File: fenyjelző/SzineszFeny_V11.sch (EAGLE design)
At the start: 203 parts, among them CN3 PIN05_2'THT', IC1 BEM_VEDO, IC2 BEM_VEDO, IC3 BEM_VEDO, IC4 BEM_VEDO, IC5 BEM_VEDO, IC6 BEM_VEDO, IC7 SCT2168SOP16, IC8 SCT2168SOP16, IC9 SCT2168SOP16, U1 MICROCHIP_PIC18F45K80-I-MLMIC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, U10 AP2625GY-HF-3SOT26, U11 AP2625GY-HF-3SOT26, U12 AP2625GY-HF-3SOT26, U13 AP2625GY-HF-3SOT26, U14 AP2625GY-HF-3SOT26, U15 AP2625GY-HF-3SOT26, U16 FDC6306P, U5 FDC6306P, U6 AP2625GY-HF-3SOT26, U7 AP2625GY-HF-3SOT26, U8 AP2625GY-HF-3SOT26, U9 AP2625GY-HF-3SOT26

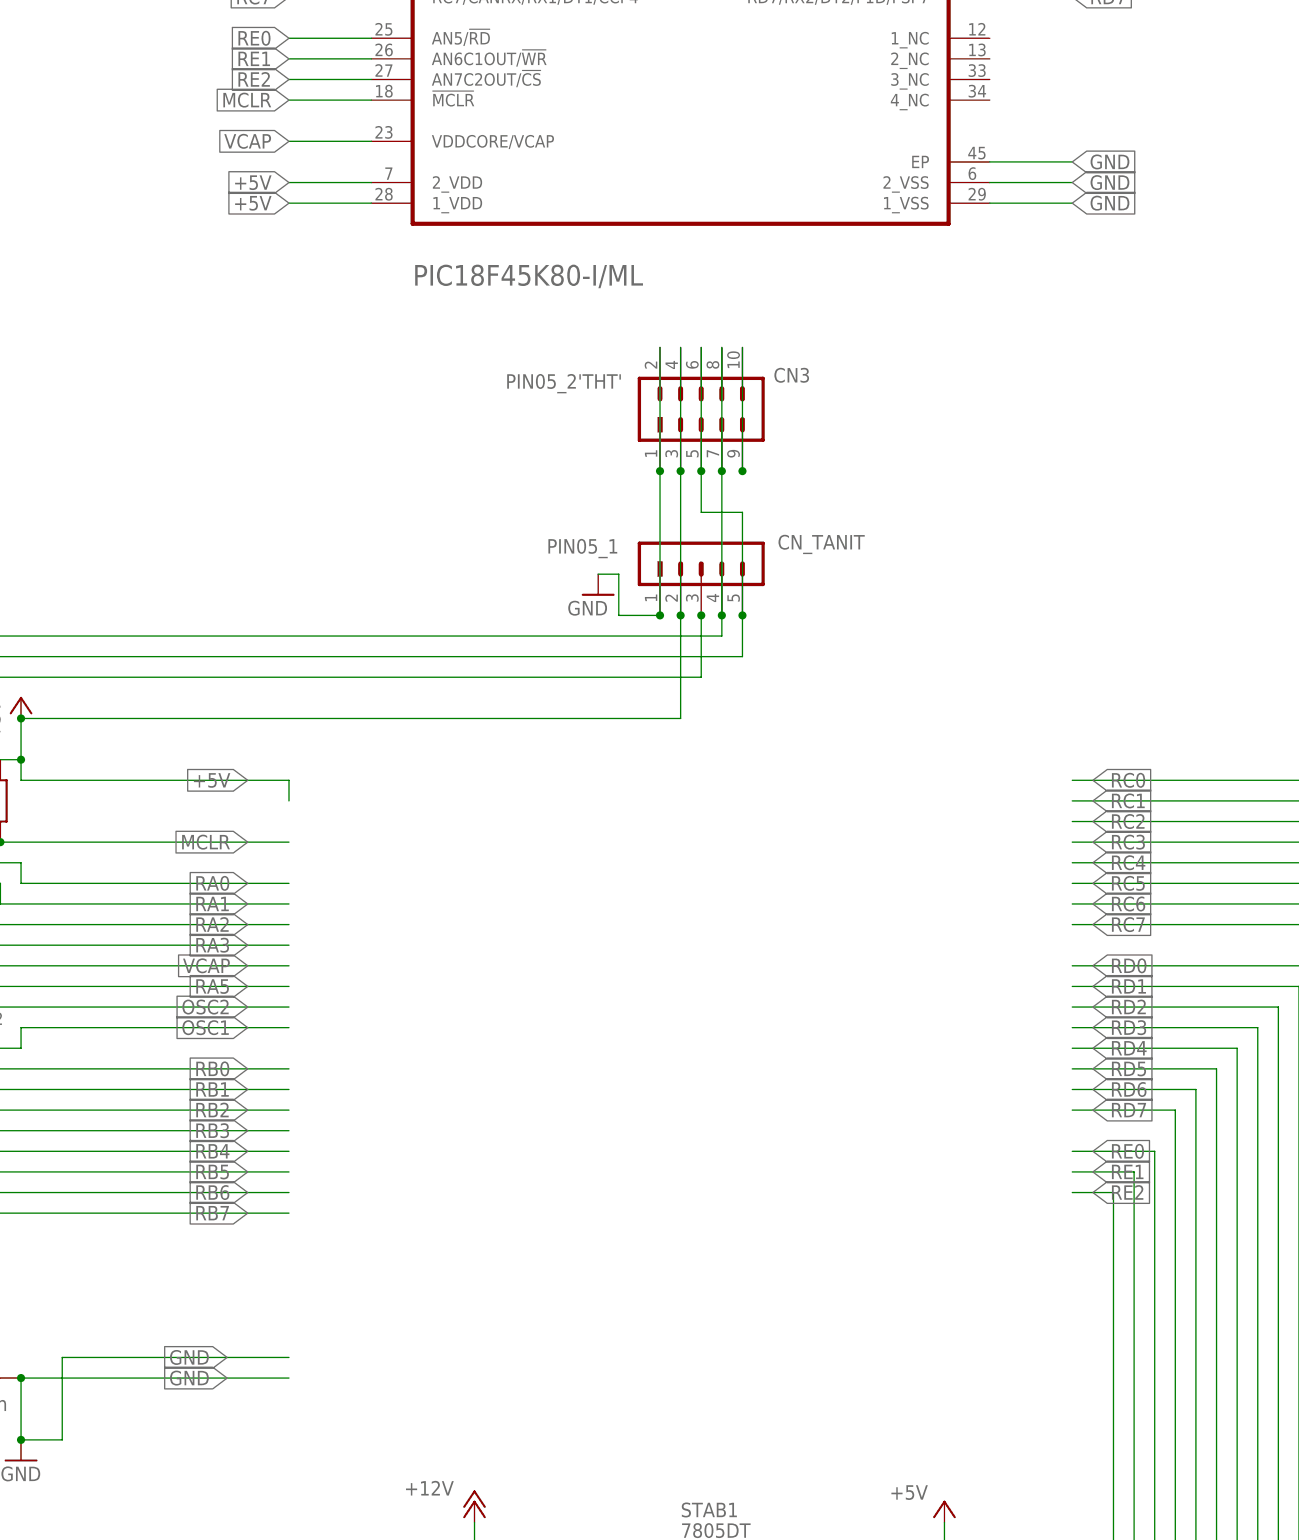
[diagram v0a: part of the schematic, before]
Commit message: fenyjelzo 90%os lett
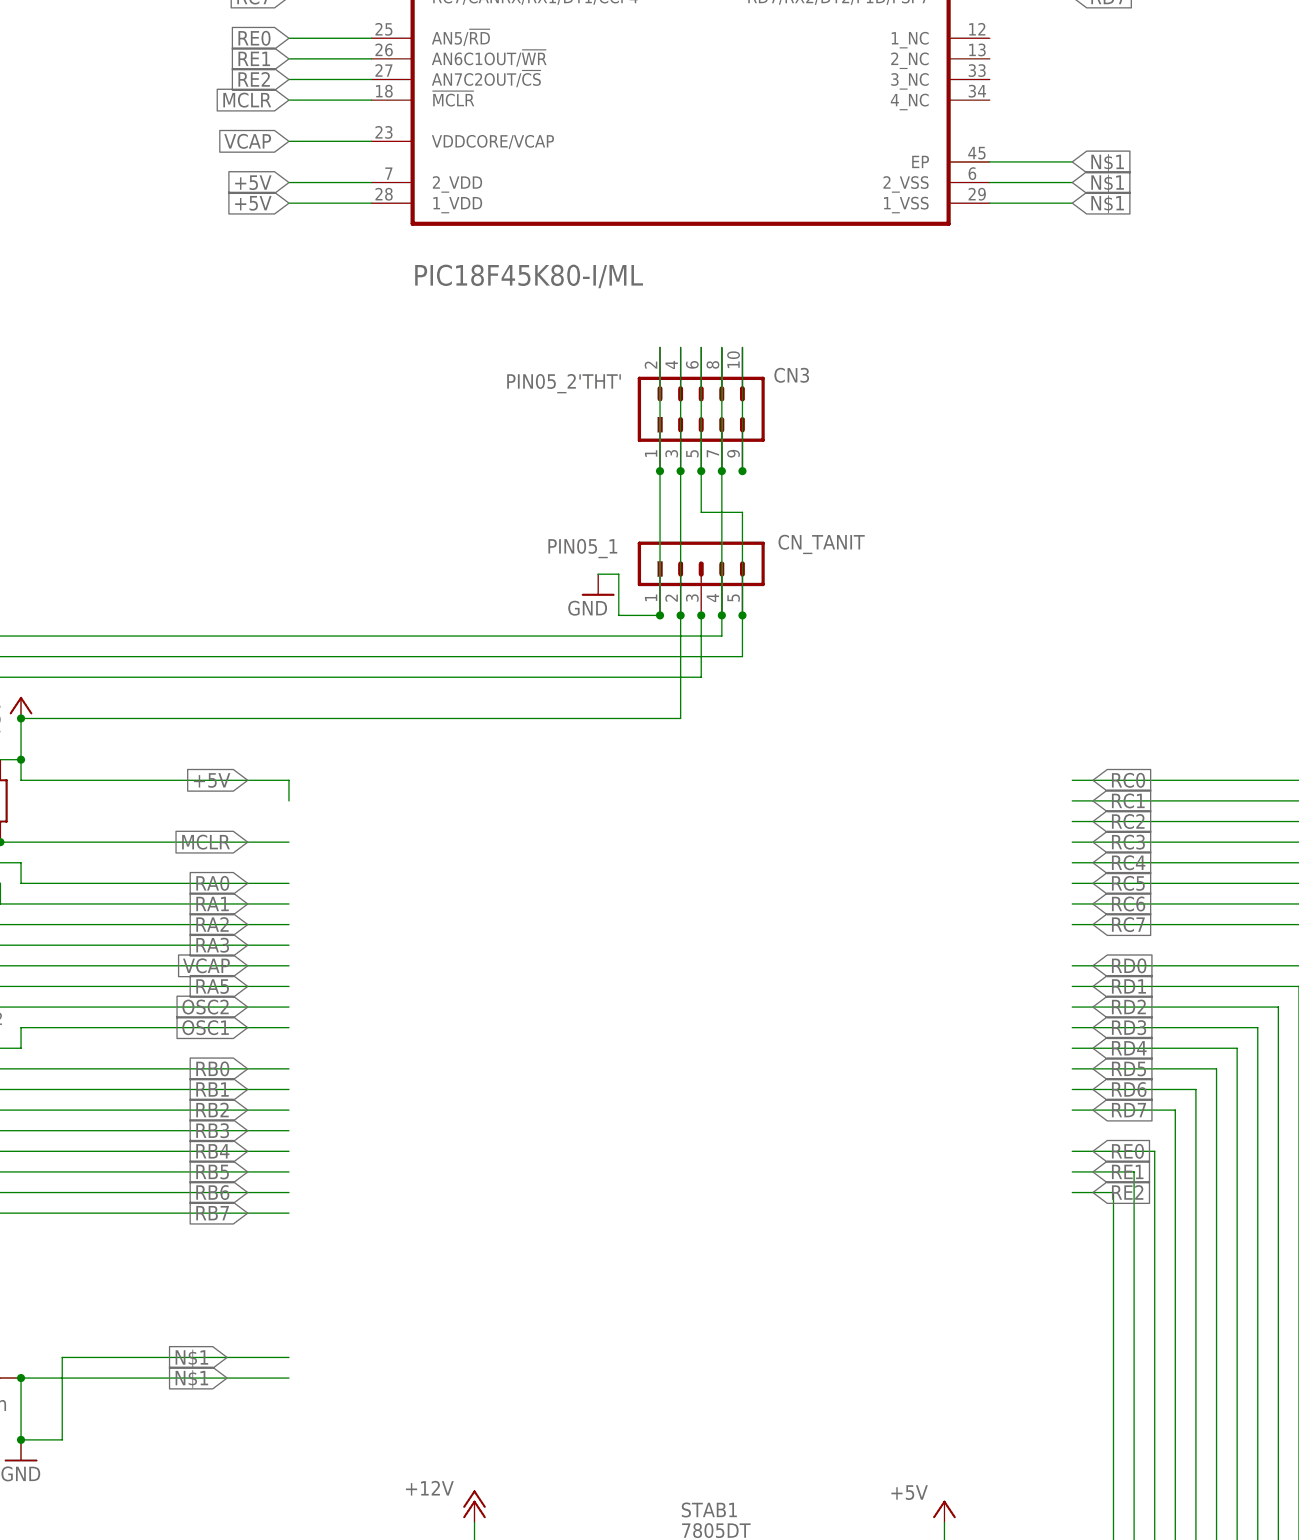
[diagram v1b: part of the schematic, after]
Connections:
- net GND renamed N$1
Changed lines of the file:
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@@
 </busses>
 <nets>
-<net name="GND" class="0">
+<net name="N$1" class="0">
 <segment>
 <pinref part="GND1" gate="1" pin="GND"/>
